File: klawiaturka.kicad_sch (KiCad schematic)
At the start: 22 parts, among them J6 Conn IN, J7 Conn OUT, SW10 SW_Push, SW11 SW_Push, SW12 SW_Push, SW13 SW_Push, SW14 SW_Push, SW15 SW_Push, SW16 SW_Push, SW17 SW_Push, SW18 SW_Push, SW3 SW_Push, SW4 SW_Push, SW5 SW_Push, SW6 SW_Push, SW7 SW_Push, SW8 SW_Push, SW9 SW_Push

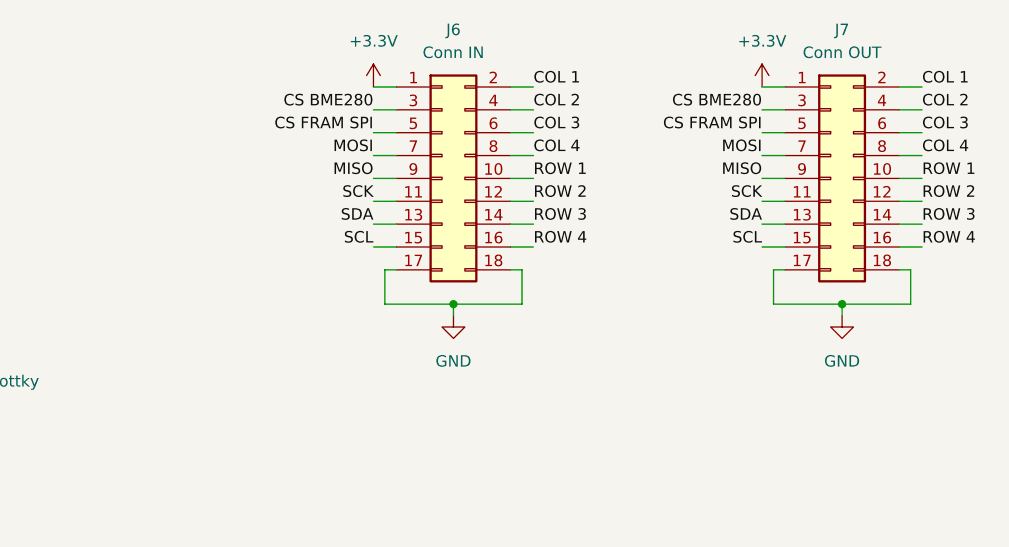
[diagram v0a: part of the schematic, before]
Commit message: awetg
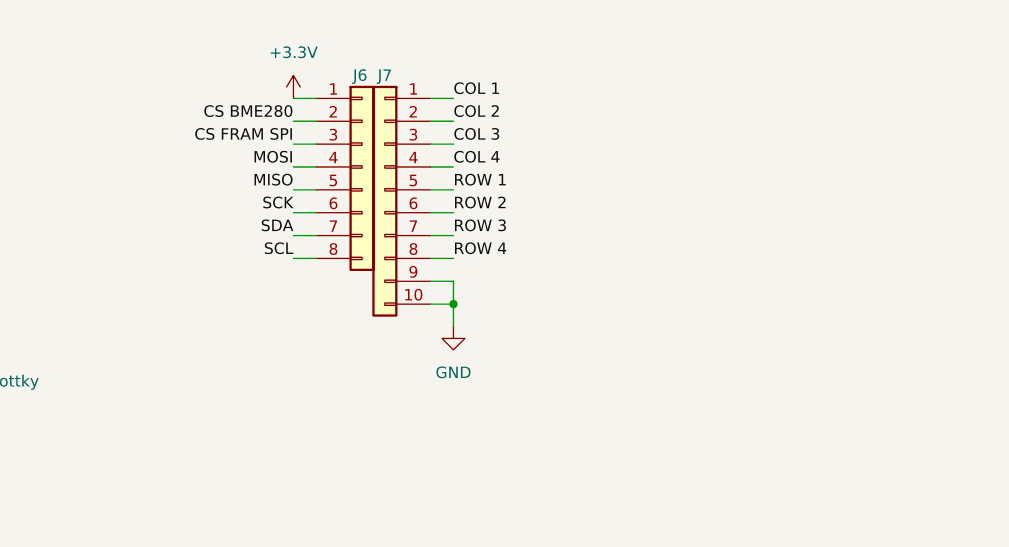
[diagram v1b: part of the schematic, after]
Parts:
- removed J6: Conn IN, Connector_PinHeader_2.54mm:PinHeader_2x09_P2.54mm_Vertical, symbol Connector_Generic:Conn_02x09_Odd_Even
- removed J7: Conn OUT, Connector_PinSocket_2.54mm:PinSocket_2x09_P2.54mm_Vertical, symbol Connector_Generic:Conn_02x09_Odd_Even
- added J6: Conn_01x08, Connector_PinHeader_2.54mm:PinHeader_1x08_P2.54mm_Vertical, symbol Connector_Generic:Conn_01x08
- added J7: Conn_01x10, Connector_PinHeader_2.54mm:PinHeader_1x10_P2.54mm_Vertical, symbol Connector_Generic:Conn_01x10
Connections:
- net +3.3V: now also J6.1 (Pin_1)
- net COL 1: now also J7.1 (Pin_1)
- net COL 2: now also J7.2 (Pin_2)
- net COL 3: now also J7.3 (Pin_3)
- net COL 4: now also J7.4 (Pin_4)
- net CS BME280: now also J6.2 (Pin_2)
- net CS FRAM SPI: now also J6.3 (Pin_3)
- net GND: now also J7.10 (Pin_10), J7.9 (Pin_9)
- net MISO: now also J6.5 (Pin_5)
- net MOSI: now also J6.4 (Pin_4)
- net ROW 1: now also J7.5 (Pin_5)
- net ROW 2: now also J7.6 (Pin_6)
- net ROW 3: now also J7.7 (Pin_7)
- net ROW 4: now also J7.8 (Pin_8)
- net SCK: now also J6.6 (Pin_6)
- net SCL: now also J6.8 (Pin_8)
- net SDA: now also J6.7 (Pin_7)
